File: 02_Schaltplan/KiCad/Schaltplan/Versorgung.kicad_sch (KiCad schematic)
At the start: 31 parts, among them J5 9V_Batt, Q2 Si2301, SW3 PWR ON/OFF, U7 TPS_54331

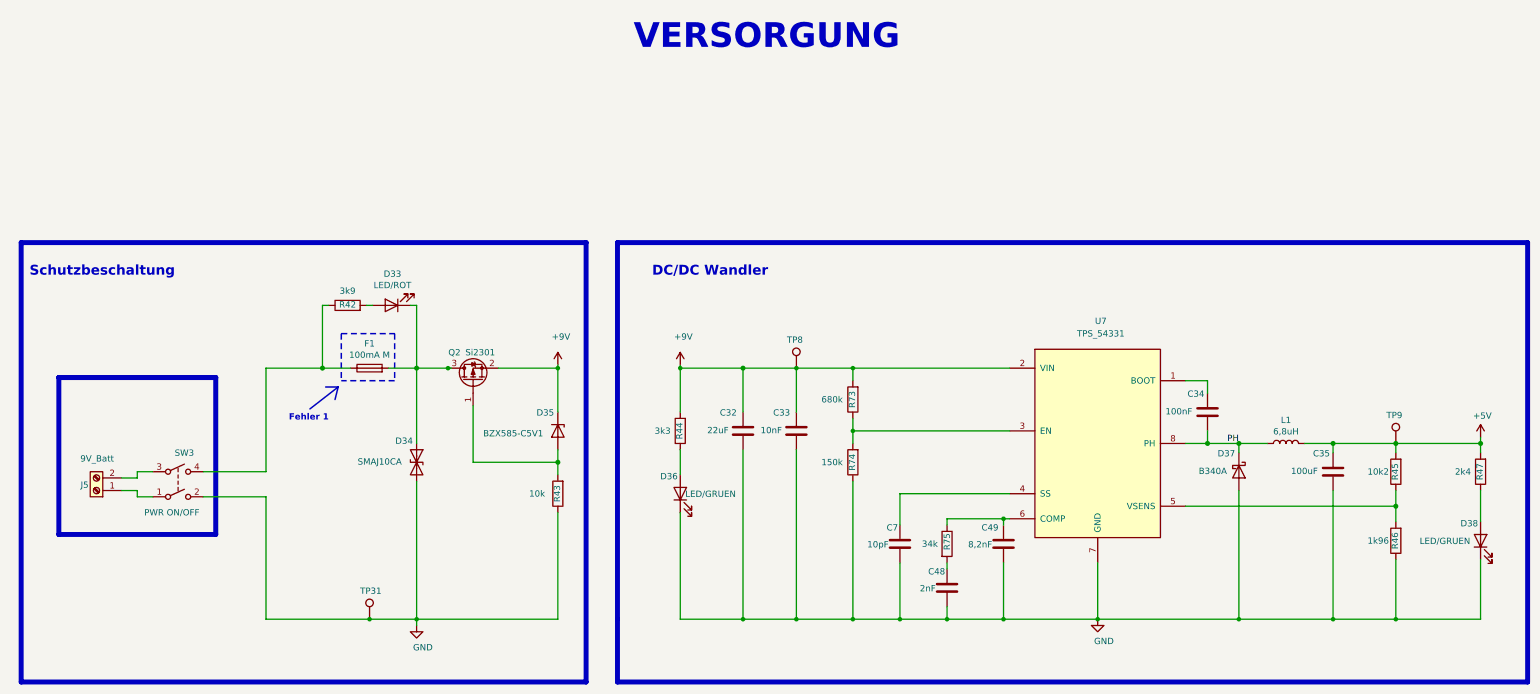
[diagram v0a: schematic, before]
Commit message: Changes
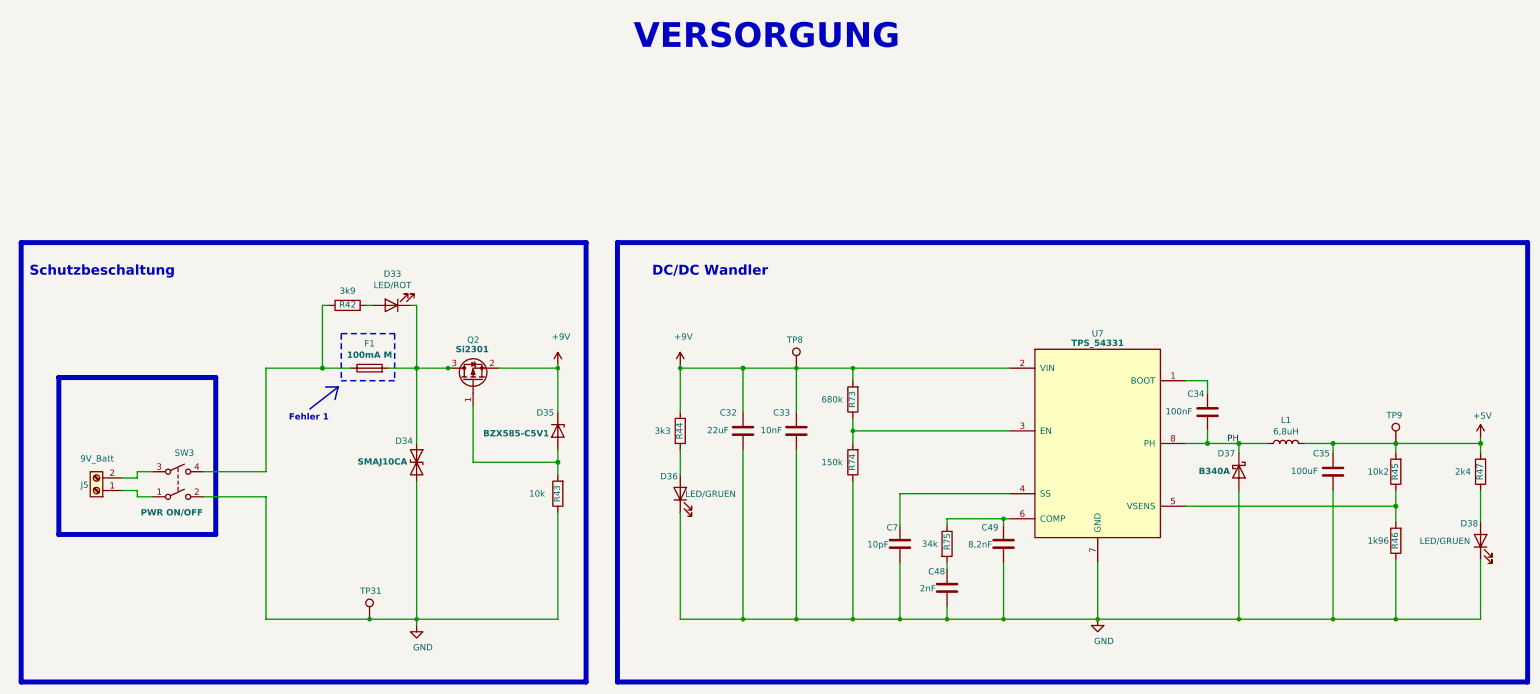
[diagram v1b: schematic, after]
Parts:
- D33: Mouser 604-APT1608LSECKJ3RV -> (none)
- D36, D38: Mouser 604-APT1608LZGCK -> (none)
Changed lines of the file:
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@@
     (in_bom yes) (on_board yes)
     (property "Reference" "F1" (id 0) (at 92.71 102.9778 90))
-    (property "Value" "100mA M" (id 1) (at 92.71 105.277 90))
+    (property "Value" "100mA M" (id 1) (at 92.71 105.277 90)
+      (effects (font (size 1.27 1.27) bold))
+    )
     (property "Footprint" "Fuse:Fuse_1812_4532Metric_Pad1.30x3.40mm_HandSolder" (id 2) (at 92.71 109.728 90)
       (effects (font (size 1.27 1.27)) hide)
@@
     )
     (property "Value" "SMAJ10CA" (id 1) (at 90.297 126.879 90)
-      (effects (font (size 1.27 1.27)) (justify left))
+      (effects (font (size 1.27 1.27) bold) (justify left))
     )
     (property "Footprint" "Diode_SMD:D_SMA_Handsoldering" (id 2) (at 102.235 127 0)
@@
     )
     (property "Value" "BZX585-C5V1" (id 1) (at 115.697 121.164 90)
-      (effects (font (size 1.27 1.27)) (justify left))
+      (effects (font (size 1.27 1.27) bold) (justify left))
     )
     (property "Footprint" "Diode_SMD:D_0805_2012Metric_Pad1.15x1.40mm_HandSolder" (id 2) (at 126.365 120.65 0)
@@
     )
     (property "Value" "B340A" (id 1) (at 260.477 128.784 90)
-      (effects (font (size 1.27 1.27)) (justify left))
+      (effects (font (size 1.27 1.27) bold) (justify left))
     )
     (property "Footprint" "Diode_SMD:D_SMA_Handsoldering" (id 2) (at 268.605 128.905 0)
@@
       (effects (font (size 1.27 1.27)) hide)
     )
-    (property "Mouser" "604-APT1608LSECKJ3RV" (id 4) (at 97.155 95.25 0)
-      (effects (font (size 1.27 1.27)) hide)
-    )
     (property "Stromaufnahme" "1mA" (id 5) (at 97.155 95.25 0)
       (effects (font (size 1.27 1.27)) hide)
@@
       (effects (font (size 1.27 1.27)) hide)
     )
-    (property "Mouser" "604-APT1608LZGCK" (id 4) (at 155.575 133.35 0)
-      (effects (font (size 1.27 1.27)) hide)
-    )
     (property "Stromaufnahme" "1mA" (id 5) (at 155.575 133.35 0)
       (effects (font (size 1.27 1.27)) hide)
@@
     )
     (property "BMK-Nr" "08-8620" (id 4) (at 317.5 142.875 0)
-      (effects (font (size 1.27 1.27)) hide)
-    )
-    (property "Mouser" "604-APT1608LZGCK" (id 4) (at 317.5 142.875 0)
       (effects (font (size 1.27 1.27)) hide)
     )
@@
     (in_bom yes) (on_board yes)
     (property "Reference" "SW3" (id 0) (at 55.245 125.095 0))
-    (property "Value" "PWR ON/OFF" (id 1) (at 52.705 137.16 0))
+    (property "Value" "PWR ON/OFF" (id 1) (at 52.705 137.16 0)
+      (effects (font (size 1.27 1.27) bold))
+    )
     (property "Footprint" "Connector_PinSocket_2.54mm:PinSocket_2x02_P2.54mm_Vertical" (id 2) (at 53.975 131.445 0)
       (effects (font (size 1.27 1.27)) hide)
@@
   (symbol (lib_id "Transistor_FET:Si2371EDS") (at 113.665 110.49 90) (unit 1)
     (in_bom yes) (on_board yes)
-    (property "Reference" "Q2" (id 0) (at 111.125 104.775 90)
-      (effects (font (size 1.27 1.27)) (justify left))
-    )
-    (property "Value" "Si2301" (id 1) (at 118.11 104.775 90)
-      (effects (font (size 1.27 1.27)) (justify left))
+    (property "Reference" "Q2" (id 0) (at 114.935 102.235 90)
+      (effects (font (size 1.27 1.27)) (justify left))
+    )
+    (property "Value" "Si2301" (id 1) (at 116.84 104.14 90)
+      (effects (font (size 1.27 1.27) bold) (justify left))
     )
     (property "Footprint" "Package_TO_SOT_SMD:SOT-23" (id 2) (at 115.57 105.41 0)
@@
   (symbol (lib_id "Kabeltester:TPS_54331") (at 240.03 123.19 0) (unit 1)
     (in_bom yes) (on_board yes)
-    (property "Reference" "U7" (id 0) (at 240.665 98.425 0))
-    (property "Value" "TPS_54331" (id 1) (at 240.665 100.965 0))
+    (property "Reference" "U7" (id 0) (at 240.03 100.965 0))
+    (property "Value" "TPS_54331" (id 1) (at 240.03 102.87 0)
+      (effects (font (size 1.27 1.27) bold))
+    )
     (property "Footprint" "Package_SO:SOIC-8_3.9x4.9mm_P1.27mm" (id 2) (at 271.78 161.29 0)
       (effects (font (size 1.27 1.27)) hide)
